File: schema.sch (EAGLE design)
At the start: 21 parts, among them Q1 2N2907

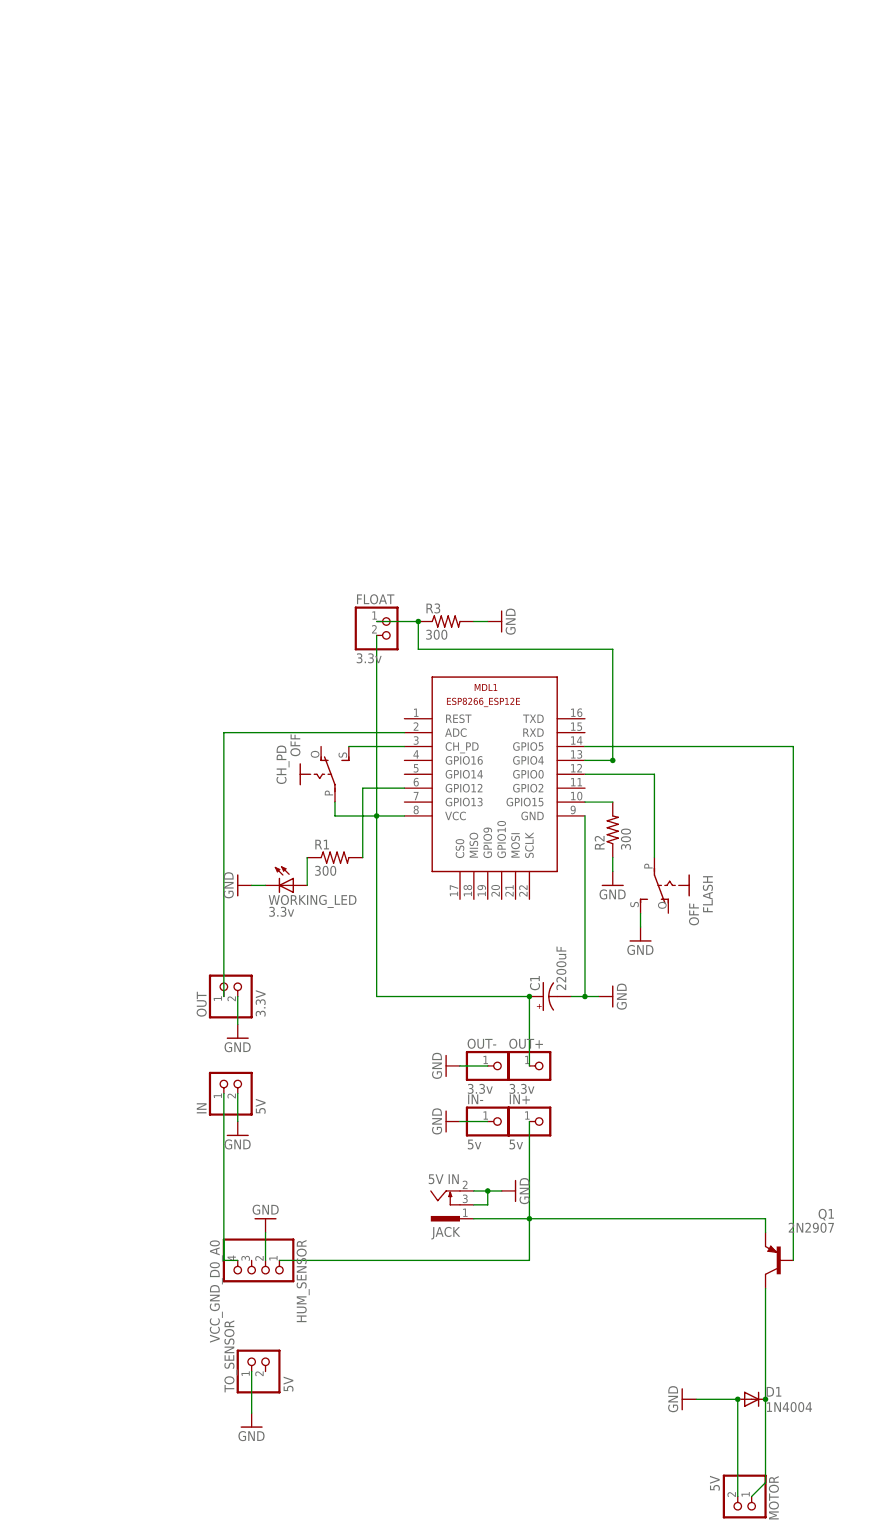
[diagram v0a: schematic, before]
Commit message: Version 2
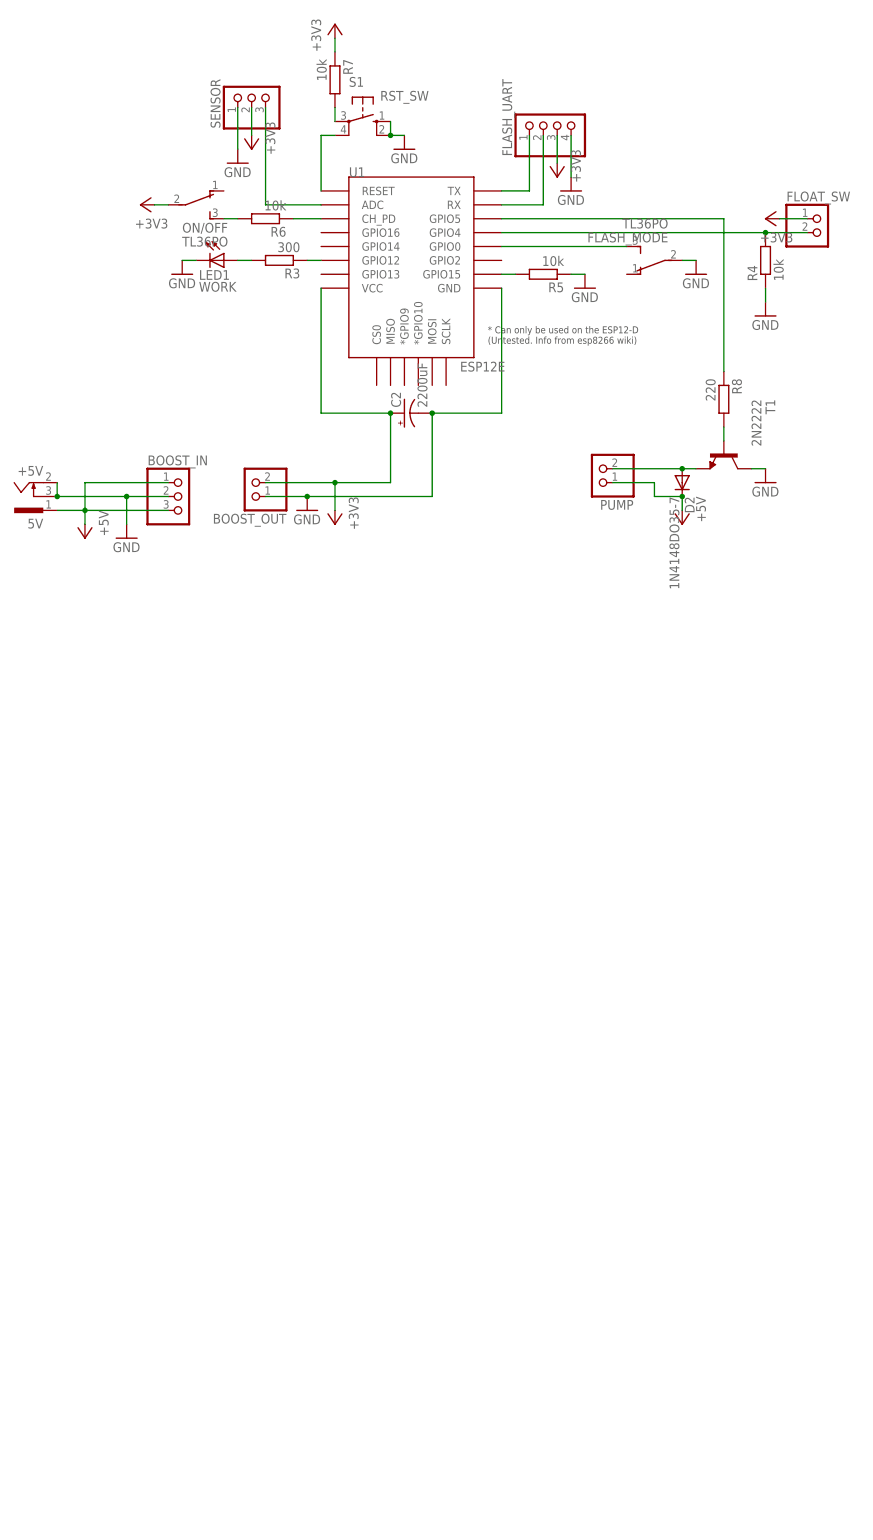
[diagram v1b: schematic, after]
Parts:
- removed C1: 2200uF, SparkFun-Capacitors:100UF-25V-20%(PTH)
- removed CH_PD, FLASH: OFF, adafruit:EG1218S
- removed D1: 1N4004, adafruit:1N4004
- removed FLOAT: 3.3v, pinhead:PINHD-1X2
- removed HUM_SENSOR: VCC_GND_D0_A0, pinhead:PINHD-1X4
- removed IN, MOTOR, TO_SENSOR: 5V, pinhead:PINHD-1X2
- removed IN+, IN-: 5v, pinhead:PINHD-1X1
- removed JACK: 5V IN, con-conrad:733989-5
- removed MDL1: ESP-12, ESP8266-ESP12E:ESP8266-12EESP8266-ESP12E
- removed OUT: 3.3V, pinhead:PINHD-1X2
- removed OUT+, OUT-: 3.3v, pinhead:PINHD-1X1
- removed Q1: 2N2907, adafruit:2N2907
- removed R1, R2: 300, adafruit:FLIPFLOP-RES
- removed WORKING_LED: 3.3v, adafruit:LED3MM
- added 5V: +5V, con-conrad:733989-5
- added BOOST_IN, SENSOR: (no value), pinhead:PINHD-1X3
- added BOOST_OUT, FLOAT_SW, PUMP: (no value), pinhead:PINHD-1X2
- added C2: 2200uF, SparkFun-Capacitors:100UF-25V-20%(PTH)
- added D2: 1N4148DO35-7, diode:1N4148DO35-7
- added FLASH_MODE, ON/OFF: TL36PO, switch:TL36PO
- added FLASH_UART: (no value), pinhead:PINHD-1X4
- added LED1: WORK, led:LED3MM
- added R4, R5, R6, R7: 10k, resistor:R-EU_0309/V
- added R8: 220, resistor:R-EU_0309/V
- added S1: RST_SW, switch-omron:10-XX
- added T1: 2N2222, transistor:2N2222
- added U1: ESP12E, esp8266modules:ESP12ESMD
- R3: device adafruit:FLIPFLOP-RES -> resistor:R-EU_0309/V
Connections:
- removed net N$1: HUM_SENSOR.4, IN.1
- removed net N$10: FLASH.P, MDL1.GPIO0
- removed net N$12: D1.C, MOTOR.1, Q1.C
- removed net N$13: FLOAT.1, MDL1.GPIO4, R3.1
- removed net N$2: MDL1.GPIO5, Q1.B
- removed net N$3: C1.+, CH_PD.P, FLOAT.2, MDL1.VCC, OUT+.1
- removed net N$4: CH_PD.S, MDL1.CH_PD
- removed net N$5: HUM_SENSOR.1, IN+.1, JACK.1, Q1.E
- removed net N$6: MDL1.ADC, OUT.1
- removed net N$7: MDL1.GPIO12, R1.2
- removed net N$8: R1.1, WORKING_LED.A
- removed net N$9: MDL1.GPIO15, R2.2
- new net +3V3: BOOST_OUT.2, C2.+, FLASH_UART.3, FLOAT_SW.1, ON/OFF.P, R7.1, SENSOR.2, U1.VCC
- new net +5V: 5V.1, BOOST_IN.1, BOOST_IN.3, D2.C, PUMP.1
- new net ADC: SENSOR.3, U1.ADC
- new net CH_PD: R6.1, U1.CH_PD
- new net CH_PD_S: ON/OFF.S, R6.2
- new net GPIO0: FLASH_MODE.S, U1.GPIO0
- new net GPIO12: R3.1, U1.GPIO12
- new net GPIO12D: LED1.A, R3.2
- new net GPIO15: R5.2, U1.GPIO15
- new net GPIO4: FLOAT_SW.2, R4.2, U1.GPIO4
- new net GPIO5: R8.1, U1.GPIO5
- new net GPIO5_T: R8.2, T1.B
- new net PUMP_GND: D2.A, PUMP.2, T1.E
- new net RST: S1.P1, U1.RESET
- new net RST_R: R7.2, S1.P
- new net RX: FLASH_UART.2, U1.RX
- new net TX: FLASH_UART.1, U1.TX
- net GND: now also 5V.2, 5V.3, BOOST_IN.2, BOOST_OUT.1, C2.-, FLASH_MODE.P, FLASH_UART.4, LED1.C, R4.1, R5.1, S1.S, S1.S1, SENSOR.1, T1.C, U1.GND; no longer C1.-, D1.A, FLASH.S, HUM_SENSOR.2, IN-.1, IN.2, JACK.2, JACK.3, MDL1.GND, MOTOR.2, OUT-.1, OUT.2, R2.1, R3.2, TO_SENSOR.1, WORKING_LED.C
